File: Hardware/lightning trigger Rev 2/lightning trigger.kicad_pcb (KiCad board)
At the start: 2 copper layers, 42.2 x 70 mm, 59 parts, among them J1 Conn_01x02, J2 Conn_02x03_Odd_Even, J3 Conn_01x04, J4 PJ-237-6A, J5 PJ-237-6A, J6 USB_OTG, J7 Conn_01x01, J8 Conn_01x01, Q1 Q_Photo_NPN, Q2 BC846B_215, SW1 SW_SPDT, U1 MCP6001, U10 MCP4532, U2 MCP4532, U3 ATMEGA328P-AU, U5 LTV-827S, U6 FS8205, U7 FS312F-G, U8 TP4056, U9 LTV-827S, Y1 Crystal

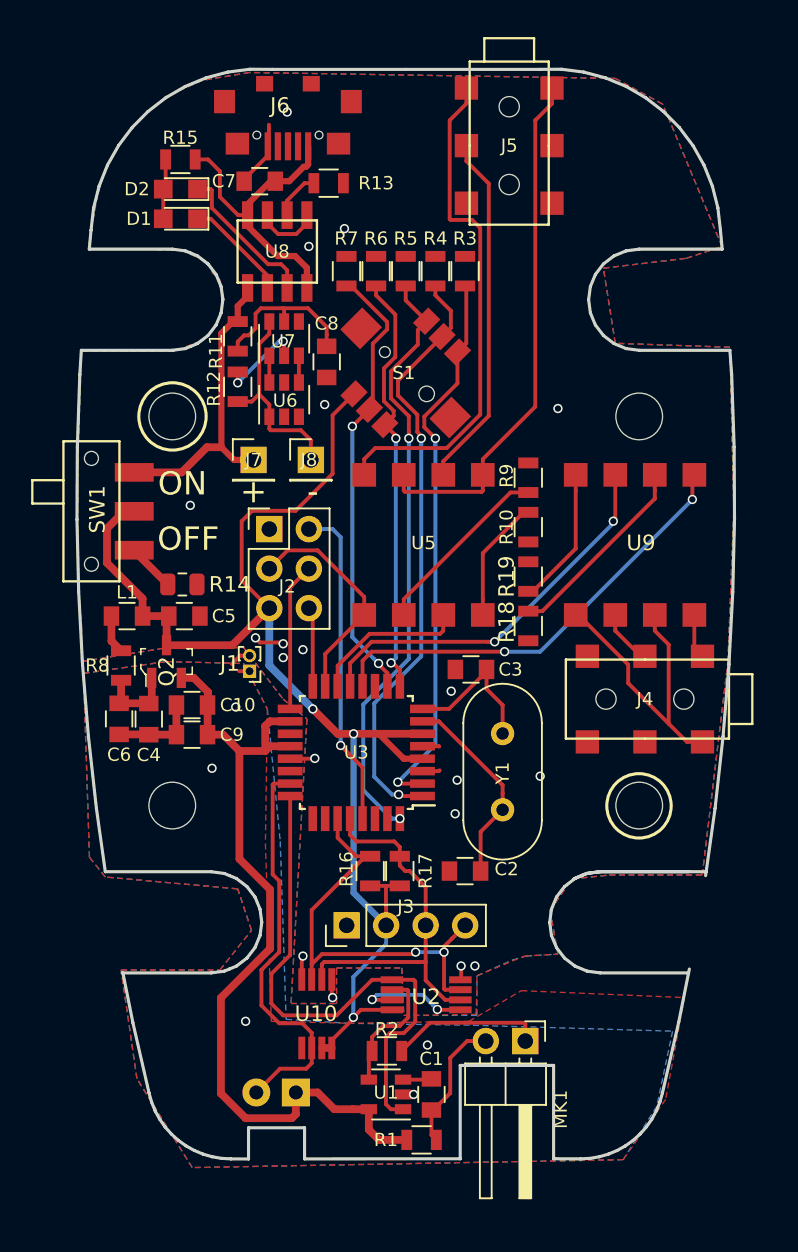
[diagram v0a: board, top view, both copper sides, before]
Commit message: Finished revision 2 of board layout
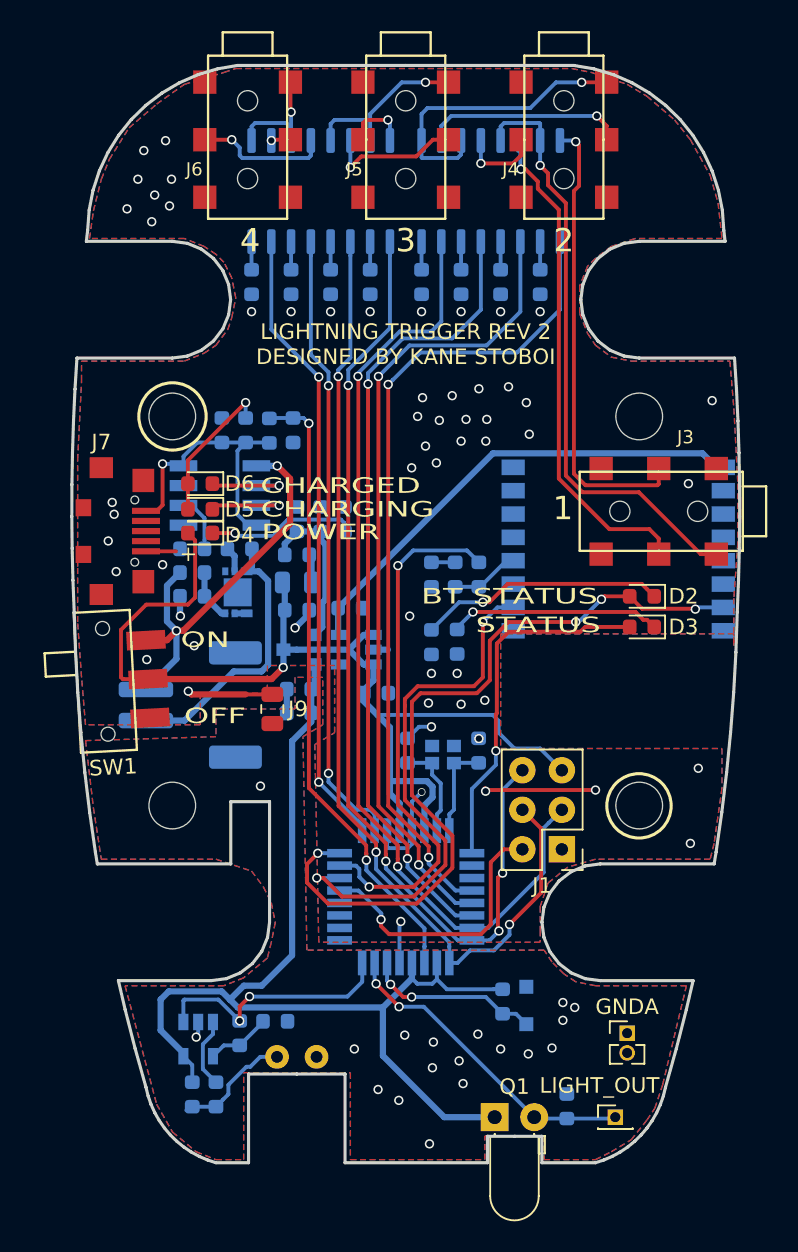
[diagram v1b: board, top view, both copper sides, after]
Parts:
- removed J2: Conn_02x03_Odd_Even, Pin_Headers:Pin_Header_Straight_2x03_Pitch2.54mm
- removed R1: 10k, Resistors_SMD:R_0805
- removed R2: 150, Resistors_SMD:R_0805
- removed S1: K1-5203UA-01, K1-5203UA-01:K1-5203UA-01
- removed U10: MCP4532, SOP:8-MSOP
- removed U9: LTV-827S, LTV-827S-TA1:LTV-827S-TA1
- added C11: 100nF, Capacitor_SMD:C_0603_1608Metric, B.Cu at (-11.8, -11.8)
- added C12: 100nF, Capacitor_SMD:C_0603_1608Metric, B.Cu at (-13.7, -1.14)
- added D3: LED, LED_SMD:LED_0603_1608Metric, F.Cu at (15.2, 0.83)
- added D4: LED, LED_SMD:LED_0603_1608Metric, F.Cu at (-13.2, -5.21)
- added D5: LED, LED_SMD:LED_0603_1608Metric, F.Cu at (-13.2, -6.73)
- added D6: LED, LED_SMD:LED_0603_1608Metric, F.Cu at (-13.2, -8.38)
- added GNDA: PinHeader_1x02_P1.27mm_Vertical, Connector_PinHeader_1.27mm:PinHeader_1x02_P1.27mm_Vertical, F.Cu at (14.2, 26.9)
- added J9: Conn_01x02, Resistor_SMD:R_0805_2012Metric, F.Cu at (-8.57, 6.10)
- added LIGHT_OUT: PinHeader_1x01_P1.27mm_Vertical, Connector_PinHeader_1.27mm:PinHeader_1x01_P1.27mm_Vertical, F.Cu at (13.5, 32.3)
- added R21: 150, Resistor_SMD:R_0603_1608Metric, B.Cu at (-2.29, -21.3)
- added R22: 150, Resistor_SMD:R_0603_1608Metric, B.Cu at (-7.37, -21.3)
- added R23: 150, Resistor_SMD:R_0603_1608Metric, B.Cu at (-4.83, -21.3)
- added R24: 150, Resistor_SMD:R_0603_1608Metric, B.Cu at (-9.91, -21.3)
- added R25: 150, Resistor_SMD:R_0603_1608Metric, B.Cu at (-13.7, -2.67)
- added R26: 2k, Resistor_SMD:R_0603_1608Metric, B.Cu at (-10.7, -4.19)
- added R27: 2k, Resistor_SMD:R_0603_1608Metric, B.Cu at (-10.3, -11.8)
- added R28: 2k, Resistor_SMD:R_0603_1608Metric, B.Cu at (-13.7, -4.19)
- added R29: 2k, Resistor_SMD:R_0603_1608Metric, B.Cu at (-3.94, -6.10)
- added U4: TLP291-4, Package_SO:SOIC-16_4.55x10.3mm_P1.27mm, B.Cu at (5.46, -27.2)
- C1, C3, C7, C8, C9: footprint Capacitors_SMD:C_0805 -> Capacitor_SMD:C_0603_1608Metric; moved to B.Cu
- C10, C4: value 1nF -> 100nF; footprint Capacitors_SMD:C_0805 -> Capacitor_SMD:C_0603_1608Metric; moved to B.Cu
- C2: value 22pF -> 10pF; footprint Capacitors_SMD:C_0805 -> Capacitor_SMD:C_0603_1608Metric; moved to B.Cu
- C5: value C -> 1nF; footprint Capacitors_SMD:C_0805 -> Capacitor_SMD:C_0603_1608Metric; moved to B.Cu
- C6: value 100nF -> 1nF; footprint Capacitors_SMD:C_0805 -> Capacitor_SMD:C_0603_1608Metric; moved to B.Cu
- D1: value Green LED -> D_Zener; footprint LEDs:LED_0805 -> Diode_SMD:SC-90A; moved to B.Cu
- D2: value Red LED -> LED; footprint LEDs:LED_0805 -> LED_SMD:LED_0603_1608Metric
- J1: value Conn_01x02 -> Conn_02x03_Odd_Even; footprint Connector_PinHeader_1.00mm:PinHeader_1x02_P1.00mm_Vertical -> Pin_Headers:Pin_Header_Straight_2x03_Pitch2.54mm
- J3: value Conn_01x04 -> SJ-2523-SMT; footprint Pin_Headers:Pin_Header_Straight_1x04_Pitch2.54mm -> PJ-237-6A:PJ-237-6A
- J4, J5: value PJ-237-6A -> SJ-2523-SMT
- J6: value USB_OTG -> SJ-2523-SMT; footprint USB_Micro:USB_Micro_C77238 -> PJ-237-6A:PJ-237-6A
- J7: value Conn_01x01 -> USB_OTG; footprint Pin_Headers:Pin_Header_Straight_1x01_Pitch2.54mm -> USB:USB_Micro_C77238
- J8: value Conn_01x01 -> Conn_01x02_Female; footprint Pin_Headers:Pin_Header_Straight_1x01_Pitch2.54mm -> Connector_JST:JST_PH_S2B-PH-SM4-TB_1x02-1MP_P2.00mm_Horizontal; moved to B.Cu
- L1: footprint Capacitors_SMD:C_0805 -> Capacitor_SMD:C_0805_2012Metric; moved to B.Cu
- MK1: footprint Pin_Headers:Pin_Header_Angled_1x02_Pitch2.54mm -> electret microphone:ELECTRET MICROPHONE; moved to B.Cu
- Q1: moved to F.Cu
- Q2: value BC846B_215 -> MMBT3904; footprint digikey-footprints:SOT-23-3 -> Package_TO_SOT_SMD:SOT-23; moved to B.Cu
- R10, R7, R9: value 150 -> 2k; footprint Resistors_SMD:R_0805 -> Resistor_SMD:R_0603_1608Metric; moved to B.Cu
- R11: value 100 -> 2k; footprint Resistors_SMD:R_0805 -> Resistor_SMD:R_0603_1608Metric; moved to B.Cu
- R12, R16, R17, R18, R19, R4, R6: footprint Resistors_SMD:R_0805 -> Resistor_SMD:R_0603_1608Metric; moved to B.Cu
- R13: value 1k -> 2k; footprint Resistors_SMD:R_0805 -> Resistor_SMD:R_0603_1608Metric; moved to B.Cu
- R14: value 1k -> 2k; footprint Resistor_SMD:R_0805_2012Metric -> Resistor_SMD:R_0603_1608Metric; moved to B.Cu
- R15: value 1k -> 160k; footprint Resistors_SMD:R_0805 -> Resistor_SMD:R_0603_1608Metric; moved to B.Cu
- R3, R5: value 150 -> 10k; footprint Resistors_SMD:R_0805 -> Resistor_SMD:R_0603_1608Metric; moved to B.Cu
- R8: value 160k -> 47; footprint Resistors_SMD:R_0805 -> Resistor_SMD:R_0603_1608Metric; moved to B.Cu
- U1, U8: moved to B.Cu
- U2: value MCP4532 -> ATMEGA328P-AU; footprint SOP:8-MSOP -> Housings_QFP:TQFP-32_7x7mm_Pitch0.8mm; moved to B.Cu
- U3: value ATMEGA328P-AU -> HM-11; footprint Housings_QFP:TQFP-32_7x7mm_Pitch0.8mm -> HM-11:HM-11; moved to B.Cu
- U5: value LTV-827S -> TLV70233_SOT23-5; footprint LTV-827S-TA1:LTV-827S-TA1 -> Package_TO_SOT_SMD:SOT-23-5; moved to B.Cu
- U6: value FS8205 -> TLP291-4; footprint TO_SOT_Packages_SMD:SOT-23-6 -> Package_SO:SOIC-16_4.55x10.3mm_P1.27mm; moved to B.Cu
- U7: value FS312F-G -> AP9211; footprint TO_SOT_Packages_SMD:SOT-23-6 -> DFN:U-DFN2030-6; moved to B.Cu
- Y1: footprint Crystals:Crystal_HC18-U_Vertical -> Crystal:Crystal_SMD_2016-4Pin_2.0x1.6mm; moved to B.Cu
- moved R3 55.7 mm to (-13.7, 30.9)
- moved D1 55.2 mm to (7.75, 25.1), turned to 0 degrees
- moved R5 54.6 mm to (10.4, 31.6)
- moved R4 50.5 mm to (-10.7, 26.9)
- moved R6 48.6 mm to (-8.38, 26.2), turned to 180 degrees
- moved D2 39.5 mm to (15.2, -1.14)
- moved R16 39.4 mm to (8.64, -21.3), turned to 270 degrees
- moved R17 38.1 mm to (3.56, -21.3), turned to 270 degrees
- moved J4 36.3 mm to (10.2, -30.5), turned to 0 degrees
- moved J3 33.3 mm to (16.3, -6.60), turned to 270 degrees
- moved R8 32.7 mm to (6.22, 24.9)
- moved R13 30.2 mm to (1.65, 1.80), turned to 90 degrees
- moved C7 27.7 mm to (-6.99, -0.25), turned to 0 degrees
- moved R15 26.5 mm to (-6.99, -3.81), turned to 0 degrees
- moved J1 23.1 mm to (10.0, 15.1)
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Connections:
- C10 pad 1: VDDA -> VIN
- C4 pad 1: Net-(C4-Pad1) -> VDDA
- C4 pad 2: GNDD -> GNDA
- C5 pad 1: VIN -> VDDA
- C5 pad 2: GNDD -> GNDA
- C6 pad 1: Net-(C4-Pad1) -> Net-(C6-Pad1)
- C7 pad 1: Net-(C7-Pad1) -> VIN
- C8 pad 1: Net-(C8-Pad1) -> Net-(C6-Pad1)
- C9 pad 1: VDDA -> 3.3V
- D1 pad 2: Net-(D1-Pad2) -> GNDA
- D2 pad 2: Net-(D1-Pad2) -> Net-(D2-Pad2)
- J1 pad 2: GNDD -> RST
- J3 pad 1: GNDD -> Net-(J3-Pad1)
- J3 pad 2: VIN -> Net-(J3-Pad2)
- J3 pad 3: SCL -> Net-(J3-Pad3)
- J3 pad 4: SDA -> (no net)
- J4 pad 4: Net-(J4-Pad4) -> (no net)
- J4 pad 5: Net-(J4-Pad5) -> (no net)
- J4 pad 6: Net-(J4-Pad6) -> (no net)
- J5 pad 4: Net-(J5-Pad4) -> (no net)
- J5 pad 5: Net-(J5-Pad5) -> (no net)
- J5 pad 6: Net-(J5-Pad6) -> (no net)
- J6 pad 1: Net-(C7-Pad1) -> Net-(J6-Pad1)
- J6 pad 4: Net-(J6-Pad4) -> (no net)
- J6 pad 5: GNDD -> (no net)
- J7 pad 1: +BATT -> VUSB
- J8 pad 1: -BAT -> +BATT
- MK1 pad 1: GNDD -> GNDA
- Q2 pad 1: Net-(C4-Pad1) -> Net-(C6-Pad1)
- R10 pad 2: GNDD -> Net-(R10-Pad2)
- R11 pad 1: Net-(C8-Pad1) -> Net-(R11-Pad1)
- R11 pad 2: +BATT -> Net-(R11-Pad2)
- R12 pad 1: -BAT -> Net-(R10-Pad2)
- R12 pad 2: Net-(R12-Pad2) -> GNDD
- R13 pad 2: Net-(R13-Pad2) -> Net-(D2-Pad1)
- R14 pad 1: Net-(R14-Pad1) -> GNDD
- R14 pad 2: GNDD -> Net-(D3-Pad1)
- R15 pad 1: Net-(C7-Pad1) -> Net-(C6-Pad1)
- R15 pad 2: Net-(D1-Pad2) -> Net-(L1-Pad1)
- R16 pad 1: VIN -> Net-(R16-Pad1)
- R16 pad 2: SDA -> GNDD
- R17 pad 1: VIN -> Net-(R17-Pad1)
- R17 pad 2: SCL -> GNDD
- R3 pad 1: LEFT -> Net-(C1-Pad2)
- R3 pad 2: GNDD -> VDDA
- R4 pad 1: CENTER -> Net-(R4-Pad1)
- R4 pad 2: GNDD -> MICROPHONE_OUT
- R5 pad 1: DOWN -> LIGHT_OUT
- R5 pad 2: GNDD -> GNDA
- R6 pad 1: UP -> GNDA
- R6 pad 2: GNDD -> Net-(R4-Pad1)
- R7 pad 1: RIGHT -> VUSB
- R7 pad 2: GNDD -> Net-(R11-Pad2)
- R8 pad 1: Net-(C4-Pad1) -> Net-(D1-Pad1)
- R8 pad 2: Net-(L1-Pad1) -> VDDA
- R9 pad 1: Net-(R9-Pad1) -> Net-(R10-Pad1)
- R9 pad 2: GNDD -> Net-(R9-Pad2)
- SW1 pad 3: Net-(R14-Pad1) -> Net-(R20-Pad1)
- U1 pad 2: GNDD -> GNDA
- U1 pad 4: Net-(R2-Pad2) -> Net-(R4-Pad1)
- U2 pad 1: GNDD -> FOCUS4
- U2 pad 2: SCL -> SHUTTER4
- U2 pad 3: SDA -> GNDD
- U2 pad 4: GNDD -> VIN
- U2 pad 5: MICROPHONE_OUT -> GNDD
- U2 pad 6: Net-(R2-Pad2) -> VIN
- U2 pad 7: GNDD -> Net-(C2-Pad1)
- U2 pad 8: VIN -> Net-(C3-Pad1)
- U3 pad 1: CENTER -> Net-(U3-Pad1)
- U3 pad 10: RIGHT -> (no net)
- U3 pad 12: SHUTTER -> GNDD
- U3 pad 13: FOCUS -> Net-(U3-Pad13)
- U3 pad 14: SHUTTER2 -> Net-(U3-Pad14)
- U3 pad 15: FOCUS2 -> Net-(D2-Pad2)
- U3 pad 16: MISO -> Net-(U3-Pad16)
- U3 pad 2: LEFT -> Net-(U2-Pad30)
- U3 pad 3: GNDD -> Net-(U3-Pad3)
- U3 pad 4: VIN -> Net-(R10-Pad1)
- U3 pad 5: GNDD -> (no net)
- U3 pad 6: VIN -> (no net)
- U3 pad 7: Net-(C2-Pad1) -> (no net)
- U3 pad 8: Net-(C3-Pad1) -> (no net)
- U3 pad 9: UP -> 3.3V
- U5 pad 1: FOCUS2 -> VIN
- U5 pad 2: Net-(R9-Pad1) -> GNDD
- U5 pad 3: SHUTTER2 -> VIN
- U5 pad 4: Net-(R10-Pad1) -> Net-(U5-Pad4)
- U5 pad 5: Net-(J5-Pad1) -> 3.3V
- U6 pad 1: -BAT -> MISO
- U6 pad 3: GNDD -> FOCUS3
- U6 pad 4: Net-(U6-Pad4) -> Net-(R23-Pad1)
- U6 pad 5: Net-(U6-Pad5) -> SHUTTER4
- U6 pad 6: Net-(U6-Pad6) -> Net-(R22-Pad1)
- U7 pad 1: Net-(U6-Pad6) -> GNDD
- U7 pad 2: Net-(R12-Pad2) -> GNDD
- U7 pad 3: Net-(U6-Pad4) -> Net-(C12-Pad1)
- U7 pad 4: Net-(U7-Pad4) -> (no net)
- U7 pad 5: Net-(C8-Pad1) -> Net-(R26-Pad2)
- U7 pad 6: -BAT -> -BATT
- U8 pad 2: Net-(R13-Pad2) -> Net-(R28-Pad2)
- U8 pad 4: Net-(C7-Pad1) -> VUSB
- U8 pad 6: Net-(D1-Pad1) -> Net-(D6-Pad1)
- U8 pad 7: Net-(D2-Pad1) -> Net-(D5-Pad1)
- U8 pad 8: Net-(C7-Pad1) -> VUSB
- Y1 pad 1: Net-(C2-Pad1) -> Net-(C3-Pad1)
- Y1 pad 2: Net-(C3-Pad1) -> Net-(C2-Pad1)
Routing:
- net FOCUS3: track 0.00 -> 63.6 mm, vias 0 -> 3
- net MISO: track 5.12 -> 62.8 mm, vias 0 -> 4
- net SHUTTER1: track 0.00 -> 52.8 mm, vias 0 -> 2
- net FOCUS1: track 0.00 -> 52.3 mm, vias 0 -> 2
- net Net-(D2-Pad2): track 0.00 -> 50.7 mm, vias 0 -> 4
- net FOCUS2: track 14.6 -> 61.7 mm, vias 0 -> 2
- net SHUTTER2: track 10.1 -> 51.5 mm, vias 0 -> 2
- net Net-(R11-Pad2): track 0.00 -> 40.4 mm, vias 0 -> 2
- net FOCUS4: track 0.00 -> 40.3 mm, vias 0 -> 2
- net SHUTTER4: track 0.00 -> 40.1 mm, vias 0 -> 2
- net CENTER: track 38.8 -> 0.00 mm, vias 2 -> 0
- net DOWN: track 38.7 -> 0.00 mm, vias 2 -> 0
- net Net-(J3-Pad1): track 0.00 -> 38.6 mm, vias 0 -> 1
- net LEFT: track 35.9 -> 0.00 mm, vias 2 -> 0
- net Net-(U2-Pad30): track 0.00 -> 34.1 mm, vias 0 -> 2
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- added copper zone on B.Cu, net GNDA
- added copper zone on F.Cu, net GNDA
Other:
- board size 42.2 x 70 mm -> 42.9 x 70.5 mm
- board text added: "1"
- board text added: "2"
- board text added: "3"
- board text added: "4"
- board text added: "BT STATUS"
- board text added: "CHARGED"
- board text added: "CHARGING"
- board text added: "LIGHTNING TRIGGER REV 2 DESIGNED BY KANE STOBOI"
- board text added: "POWER"
- board text added: "STATUS"
- board text removed: "Lightning Trigger v1"
